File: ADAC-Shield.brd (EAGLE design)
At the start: 100 x 80 mm, 58 parts, among them U1 ARDUINO-MEGAFULL, U2 LM358D

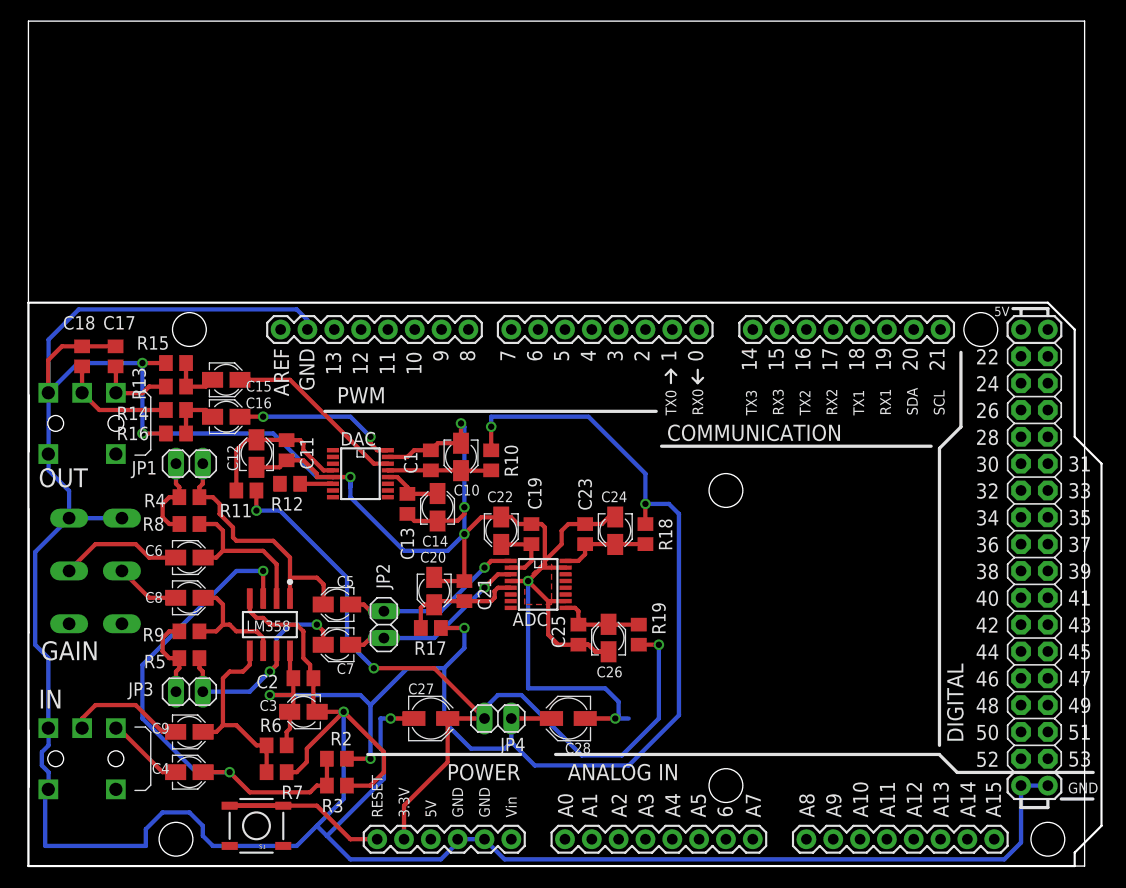
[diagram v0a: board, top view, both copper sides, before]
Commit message: Board layout finished for v0.1
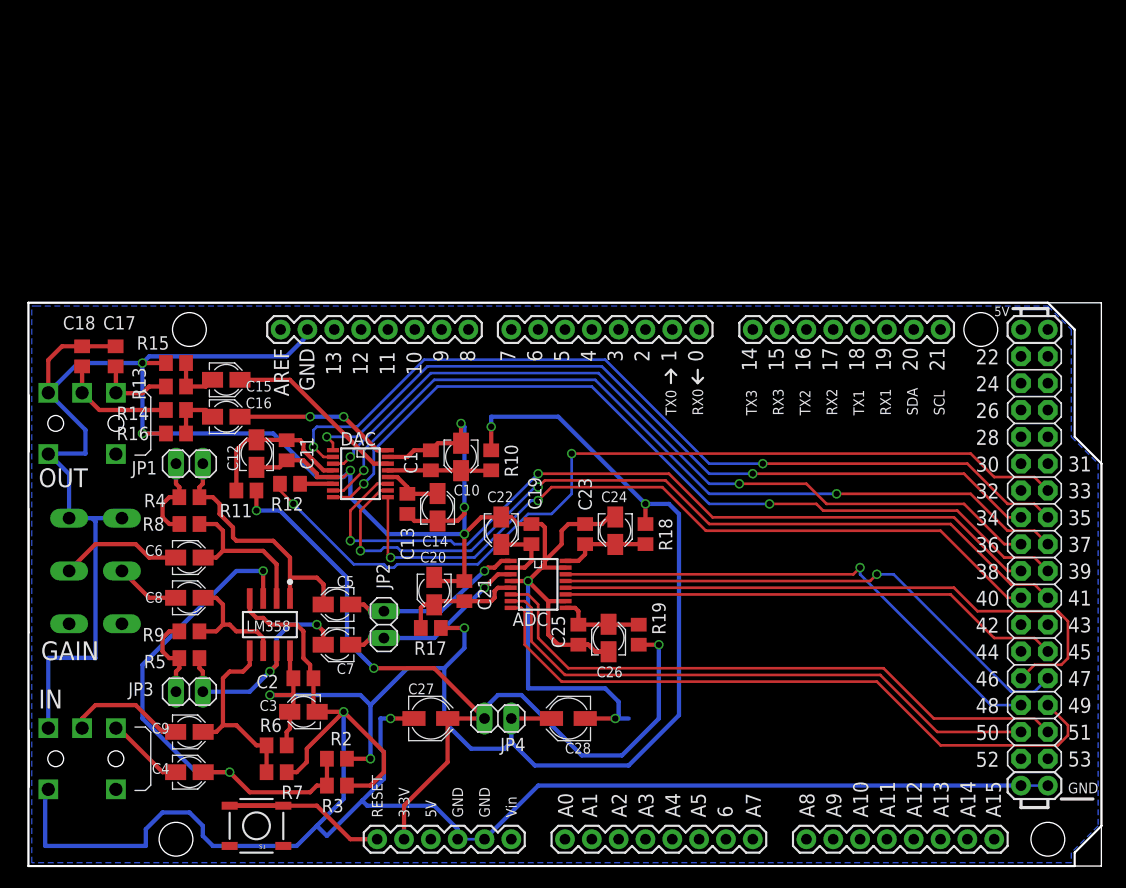
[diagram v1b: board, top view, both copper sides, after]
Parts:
- U1: device SparkFun-Boards:ARDUINO_MEGA -> SparkFun-Boards_modified:ARDUINO_MEGA
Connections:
- net ADC_BCK: now also U1.45
- net ADC_DATAO: now also U1.47
- net ADC_MSSEL: now also U1.48
- net ADC_PWON: now also U1.50
- net ADC_SFOR: now also U1.51
- net ADC_SYSCLK: now also U1.49
- net ADC_WS: now also U1.46
- net DAC_BCK: now also U1.34
- net DAC_DATAI: now also U1.36
- net DAC_DEEM: now also U1.40
- net DAC_MUTE: now also U1.39
- net DAC_PCS: now also U1.41
- net DAC_SFOR0: now also U1.38
- net DAC_SFOR1: now also U1.37
- net DAC_SYSCLK: now also U1.33
- net DAC_WS: now also U1.35
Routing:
- net DAC_SYSCLK: track 0.00 -> 84.5 mm, vias 0 -> 2
- net DAC_WS: track 0.00 -> 82.3 mm, vias 0 -> 2
- net DAC_MUTE: track 0.00 -> 80.6 mm, vias 0 -> 2
- net DAC_PCS: track 0.00 -> 79.9 mm, vias 0 -> 2
- net DAC_SFOR1: track 0.00 -> 79.6 mm, vias 0 -> 2
- net DAC_SFOR0: track 0.00 -> 77.7 mm, vias 0 -> 2
- net DAC_BCK: track 0.00 -> 75.9 mm, vias 0 -> 2
- net DAC_DATAI: track 0.00 -> 75.6 mm, vias 0 -> 2
- net DAC_DEEM: track 0.00 -> 72.6 mm, vias 0 -> 2
- net ADC_SYSCLK: track 0.00 -> 64.1 mm
- net ADC_SFOR: track 0.00 -> 58.1 mm
- net ADC_WS: track 0.00 -> 57.6 mm
- net ADC_PWON: track 0.00 -> 55.3 mm
- net ADC_DATAO: track 0.00 -> 51.1 mm, vias 0 -> 1
- net ADC_MSSEL: track 0.00 -> 49.1 mm, vias 0 -> 1
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- added copper zone on layer 16, net GND
- removed copper zone on layer 1, net GND
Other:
- board size 100 x 80 mm -> 101.6 x 53.3 mm
